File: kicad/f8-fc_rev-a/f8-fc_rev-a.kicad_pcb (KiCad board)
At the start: 4 copper layers, 34.7 x 34.7 mm, 114 parts, among them J1 Battery, J10 USART1, J11 USART2, J12 FC-ESC con, J13 Motors2, J14 UART4, J15 USART6, J16 I2C, J17 I2C, J18 I2C, J19 Debug, J2 M1, J3 M2, J4 M3, J5 M4, J6 M5, J7 M6, J8 M7, J9 M8, Q1 PMOS, Q2 2300A, Q3 2300A, Q4 2300A, Q5 2300A, Q6 2300A, Q7 2300A, Q8 2300A, Q9 2300A, SW1 SW_SPST, U1 STM32F405RGT6, U13 W25Q128JVS, U14 INA180A3, U2 BMP388, U3 BMI270, U4 TPS62172DSG, U5 GT-USB-7010AN, Y1 8 MHz

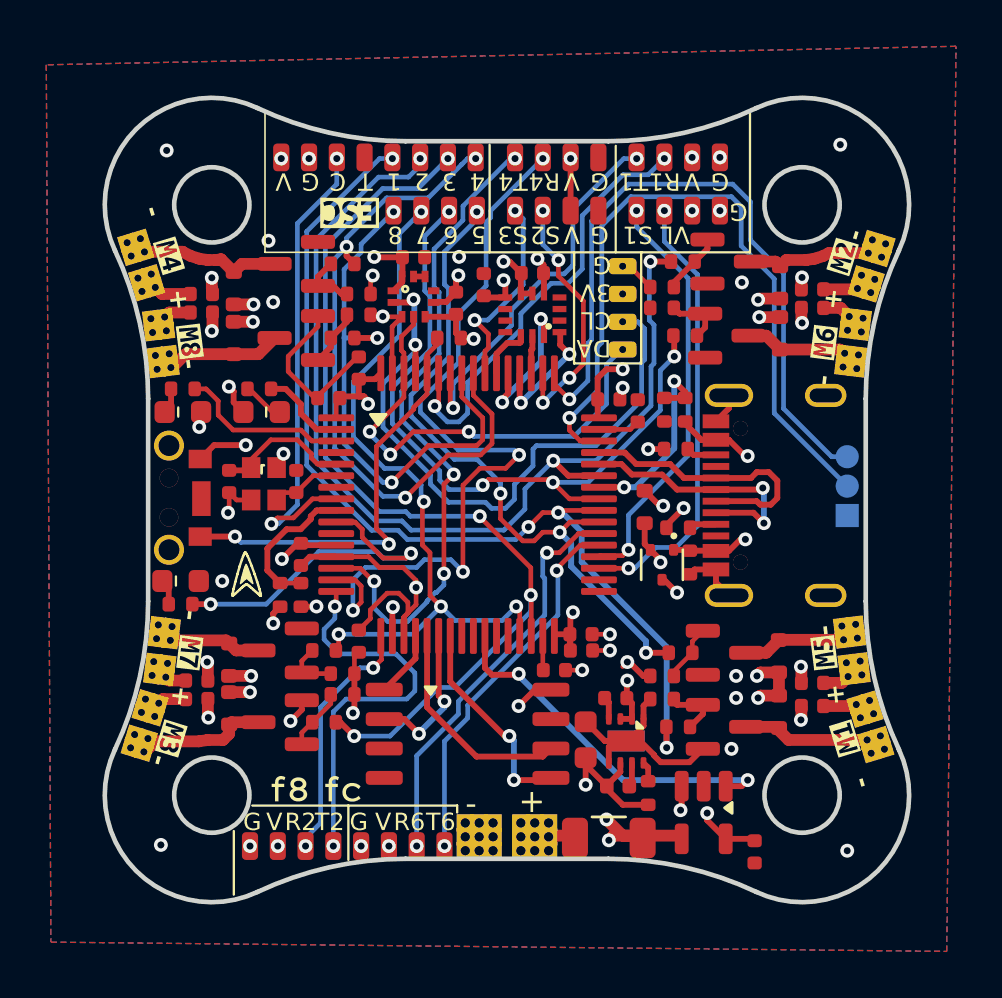
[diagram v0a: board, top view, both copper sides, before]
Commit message: rev. A is ready to order!
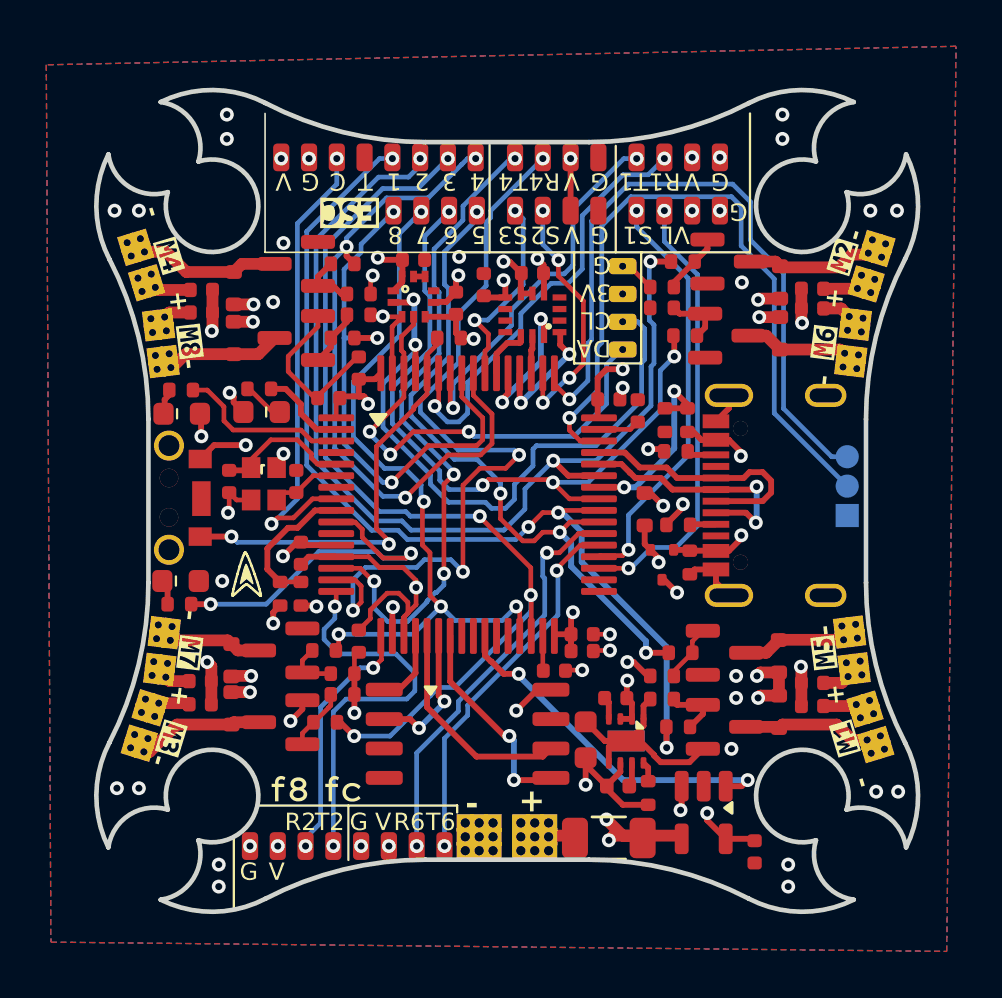
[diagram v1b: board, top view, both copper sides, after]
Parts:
- moved R2 0.46 mm to (175.9, 119.3)
- moved R3 0.45 mm to (174.9, 119.3)
- moved C19 0.27 mm to (154.8, 131.6)
- moved C20 0.18 mm to (154.9, 113.7)
- moved C23 0.15 mm to (154.8, 130.6)
- moved R10 0.12 mm to (175.5, 123.9)
- moved C5 0.11 mm to (164.1, 112.4)
- moved D11 0.10 mm to (156.2, 129.7)
- moved D4 0.10 mm to (174.1, 123.2)
- moved R9 0.10 mm to (175.4, 120.7)
- moved D7 0.10 mm to (156.2, 131.8)
- moved D2 0.09 mm to (154.1, 119.1)
- moved R5 0.09 mm to (154.0, 118.0)
- moved C16 0.05 mm to (159.2, 125.1)
- moved R18 0.05 mm to (160.2, 132.4)
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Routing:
- net GND: track 58.7 -> 62.5 mm, vias 45 -> 53
- net +3.3V: track 111.3 -> 108.7 mm
- net VBUS: track 16.1 -> 15.1 mm
- net USB+: track 12.0 -> 11.2 mm
- net USB-: track 11.4 -> 10.8 mm
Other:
- board size 34.7 x 34.7 mm -> 35.5 x 35.5 mm
- board text added: "GND"
- board text added: "SCK"
- board text added: "SWD"
